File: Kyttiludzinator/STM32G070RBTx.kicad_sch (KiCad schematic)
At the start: 36 parts, among them IC201 STM32G070RBT6, J201 Conn_02x07_Odd_Even, J202 Conn_02x14_Odd_Even, J203 Conn_02x14_Odd_Even, J205 Conn_01x08, SW201 SW_Push, SW202 SW_Push, SW203 SW_Push, SW204 SW_Push, Y201 16MHz

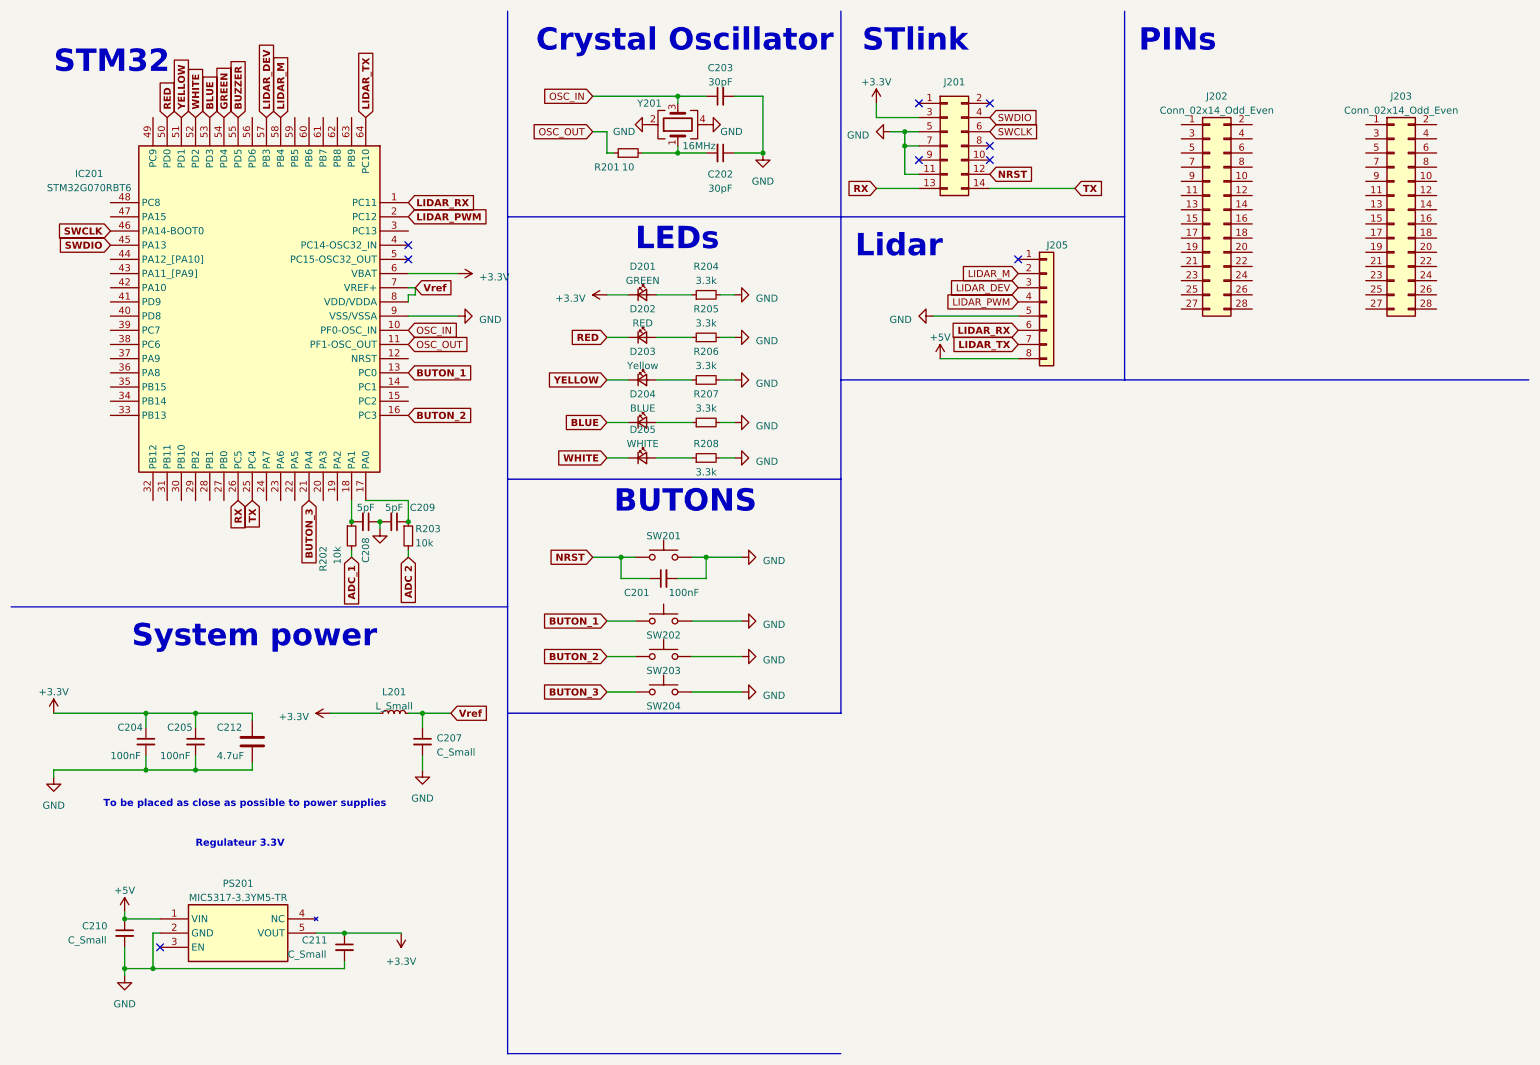
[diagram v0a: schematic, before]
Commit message: version Antoine 21-09-23
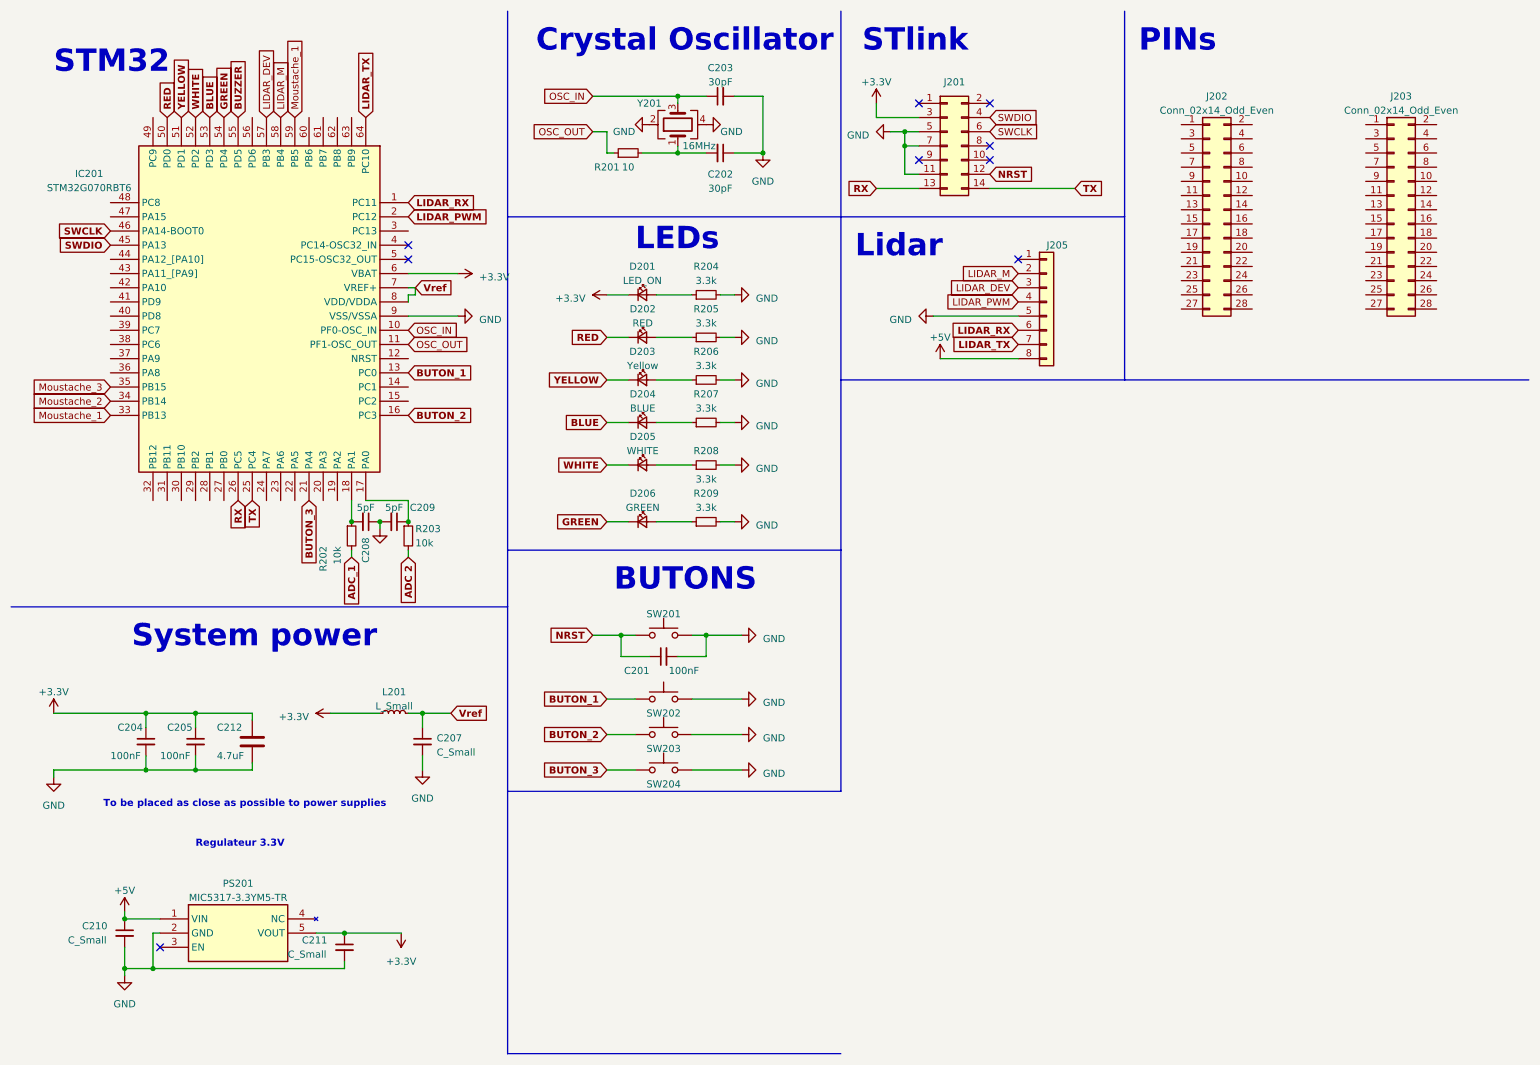
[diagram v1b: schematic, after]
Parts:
- added D206: GREEN, symbol Device:LED_Small
- added R209: 3.3k, symbol Device:R_Small
- D201: value GREEN -> LED_ON
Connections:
- net GND: now also R209.2
- net GREEN: now also D206.1 (K)
- net Moustache_1: now reaches IC201.33 (PB13)
- net Moustache_1: now also IC201.59 (PB5)
- net Moustache_2: now reaches IC201.34 (PB14)
- net Moustache_3: now reaches IC201.35 (PB15)
- new net: D206.2 (A), R209.1
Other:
- moved on the sheet: C201, D205, R208, SW201, SW202, SW203, SW204
